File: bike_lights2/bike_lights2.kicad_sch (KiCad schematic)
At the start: 36 parts, among them J2 LED, J3 B+, P1 USB_C_Plug_USB2.0, SW1 TL49, U1 TL431DBZ, U3 MIC2289, U4 MCP6002-xMS, U5 MCP73831-2-ADI/OT

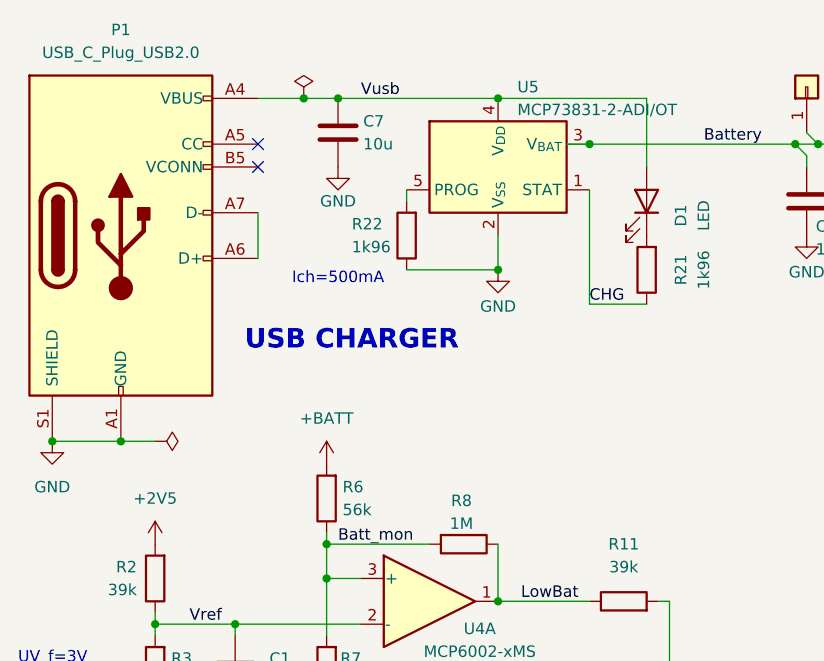
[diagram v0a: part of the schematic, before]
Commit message: a
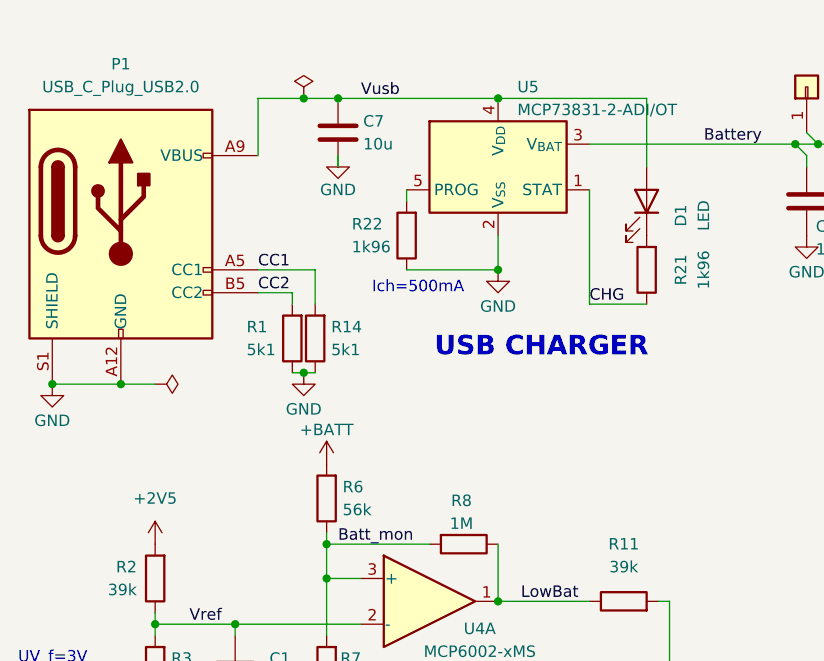
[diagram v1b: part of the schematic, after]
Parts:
- added R1, R14: 5k1, Resistor_SMD:R_0603_1608Metric, symbol Device:R
- J2: footprint Connector_PinHeader_2.54mm:PinHeader_1x02_P2.54mm_Vertical -> footprints:JST_PH_1x02_P2.0-2.5mm_Vertical
- P1: symbol Connector:USB_C_Plug_USB2.0 -> Connector:USB_C_Receptacle_PowerOnly_6P
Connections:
- net GND: now also R1.1, R14.1; no longer P1.A1 (GND), P1.B1 (GND)
- net Vusb: no longer P1.A4 (VBUS), P1.B4 (VBUS)
- net CC1: now reaches P1.A5 (CC1)
- net CC1: now also R14.2
- net CC2: now reaches P1.B5 (CC2)
- net CC2: now also R1.2
- no-connect marks 4 -> 2
